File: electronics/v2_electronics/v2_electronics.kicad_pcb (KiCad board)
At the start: 2 copper layers, 37 parts, among them J1 Main Connector, J2 Main Power, J3 12-6V Converter, J4 Controller Battery Connector, J5 Depth Sensor, K1 G5Q-1 5V, K2 G5Q-1 5V, K3 G5Q-1 5V, K4 G5Q-1 5V, K5 T9AS1D12, K6 G5Q-1A 12V, Q1 BC547, Q2 BC547, Q3 BC547, Q4 BC547, Q5 BC547, Q6 BC557, U1 raspberry_pi_pico, U2 mpu6050_breakout

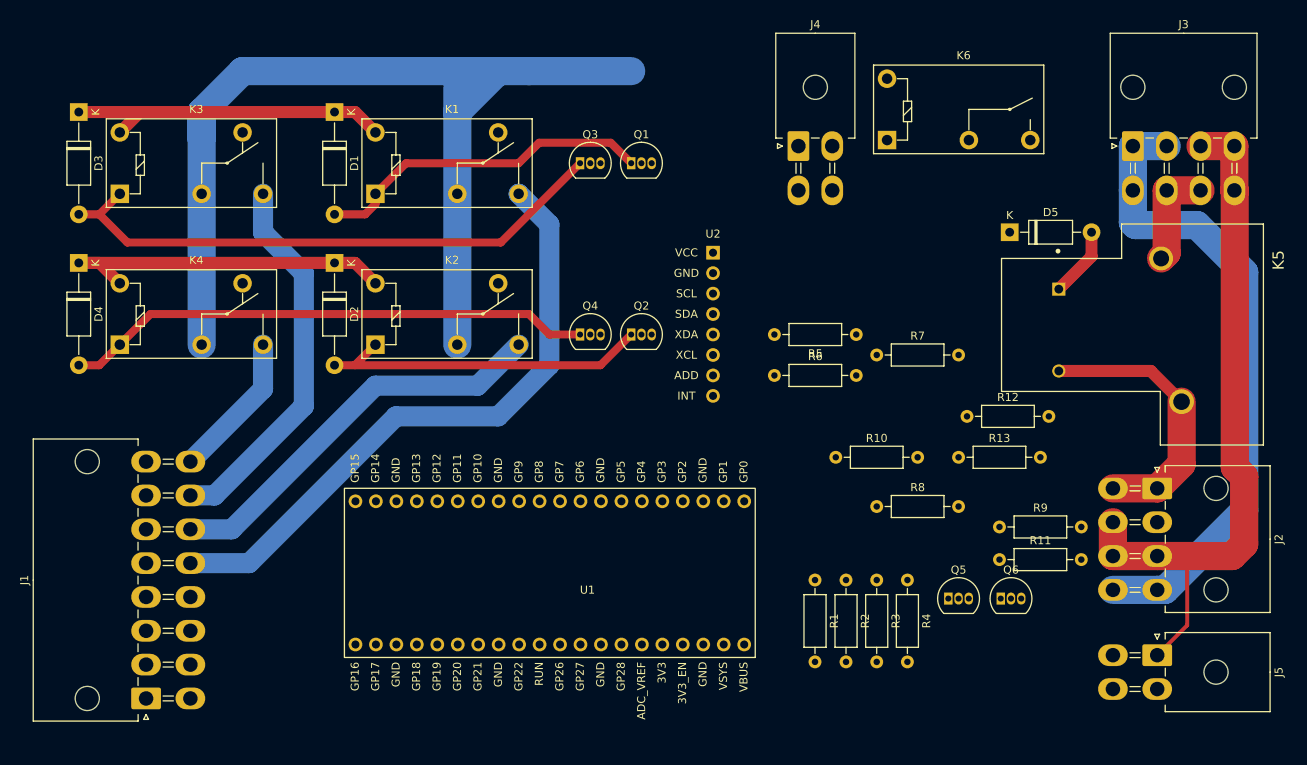
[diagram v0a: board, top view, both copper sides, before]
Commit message: do most of the work on v2 pcb
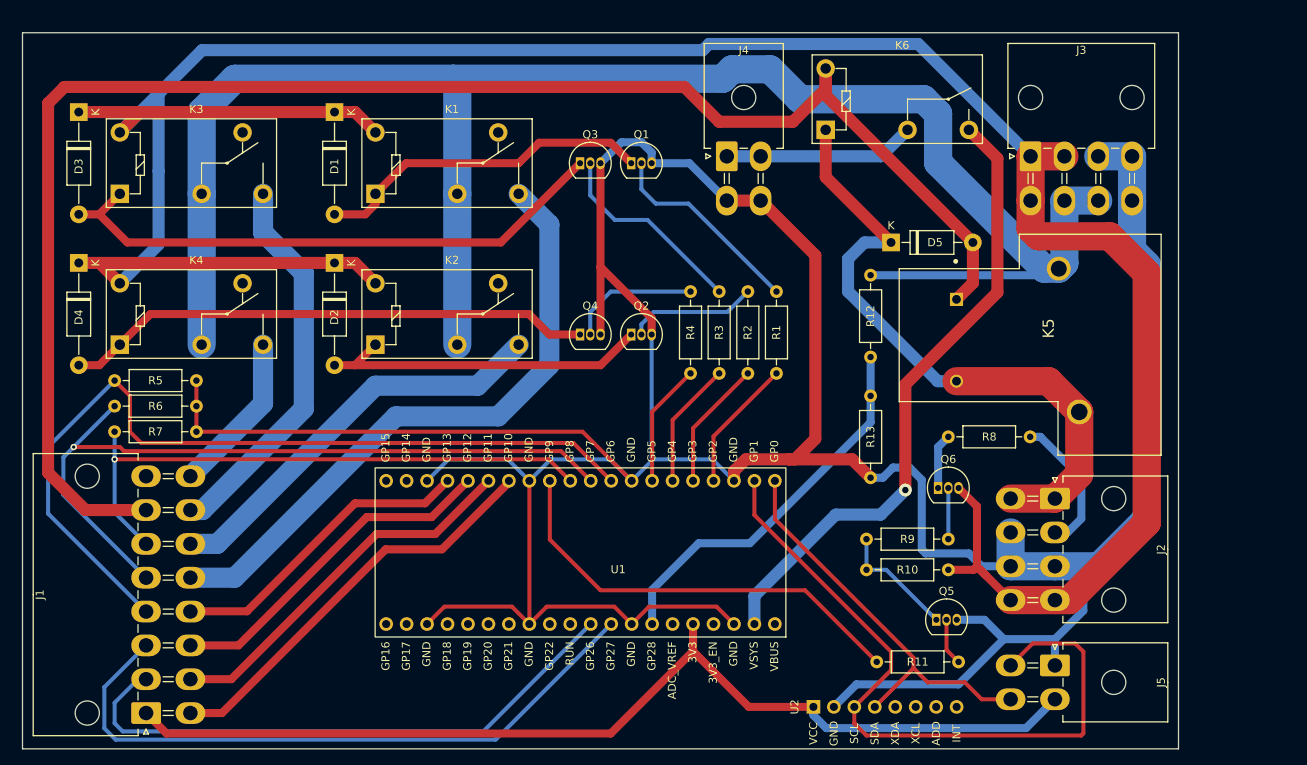
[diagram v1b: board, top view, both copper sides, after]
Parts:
- moved R7 85.0 mm to (139.1, 107.3), turned to 180 degrees
- moved R5 82.1 mm to (139.1, 101.0)
- moved R6 71.9 mm to (139.1, 104.1), turned to 180 degrees
- moved U2 52.7 mm to (223.3, 141.5), turned to 90 degrees
- moved R4 44.8 mm to (200.4, 89.9)
- moved R3 40.8 mm to (204.0, 89.9)
- moved R2 37.8 mm to (207.5, 89.9)
- moved R1 36.1 mm to (211.1, 89.9)
- moved R11 19.8 mm to (223.5, 135.9)
- moved R10 19.8 mm to (232.4, 124.5), turned to 180 degrees
- moved R9 16.6 mm to (222.2, 120.7)
- moved Q6 15.8 mm to (231.1, 114.3)
- moved D5 14.8 mm to (225.3, 83.8)
- moved R12 14.1 mm to (222.8, 98.0), turned to 90 degrees
- moved J2 12.8 mm to (245.6, 115.6)
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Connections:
- Q6 pad 1: Net-(Q6-Pad1) -> /External LED
- Q6 pad 2: /External LED -> Net-(R9-Pad2)
- R9 pad 2: Net-(Q6-Pad1) -> Net-(R9-Pad2)
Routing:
- net GND: track 89.1 -> 451.8 mm
- net /MC:7: track 8.75 -> 200.4 mm
- net /+6V: track 166.1 -> 335.5 mm
- net /3V3: track 0.00 -> 127.5 mm
- net /GP6: track 0.00 -> 106.5 mm
- net /GP7: track 0.00 -> 94.1 mm, vias 0 -> 1
- net /GP1: track 0.00 -> 88.9 mm
- net /+12V: track 139.1 -> 221.2 mm
- net /GP27: track 0.00 -> 81.9 mm
- net /VSYS: track 0.00 -> 78.6 mm, vias 0 -> 1
- net /Blow Button: track 0.00 -> 73.2 mm, vias 0 -> 1
- net /GP26: track 0.00 -> 72.7 mm
- net /GP9: track 0.00 -> 54.2 mm
- net /GP10: track 0.00 -> 51.6 mm
- net /GP0: track 0.00 -> 50.8 mm
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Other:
- board outline added: 143.5 x 88.9 mm
